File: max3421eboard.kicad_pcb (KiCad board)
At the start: 2 copper layers, 41 x 49 mm, 32 parts, among them J1 USB A, J2 USB MicroB, J3 1x10, J4 1x8, J5 1x8, J6 1x3, J7 Conn_01x04, U1 MAX3421E, U2 LP2985-3.3, U3 STMPS2141STR, Y1 12MHz

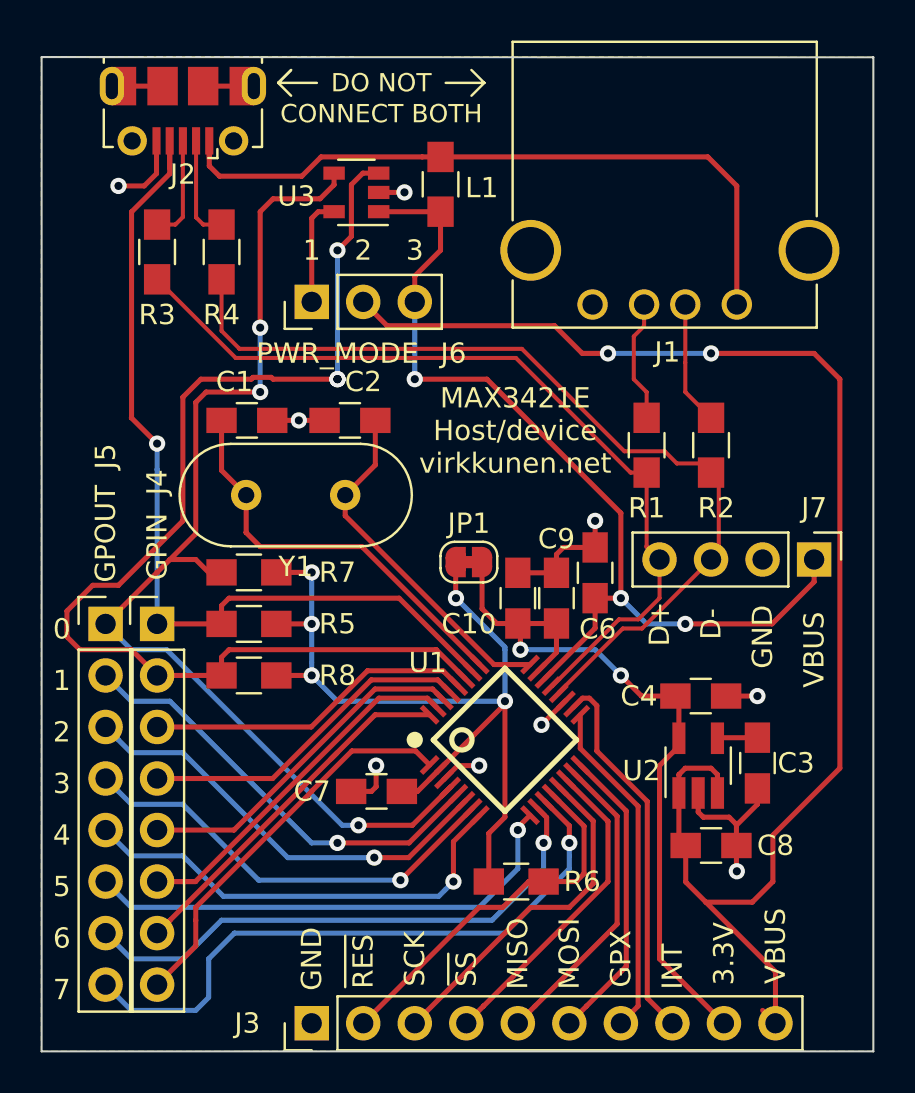
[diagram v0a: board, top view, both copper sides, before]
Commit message: Fix the board layout
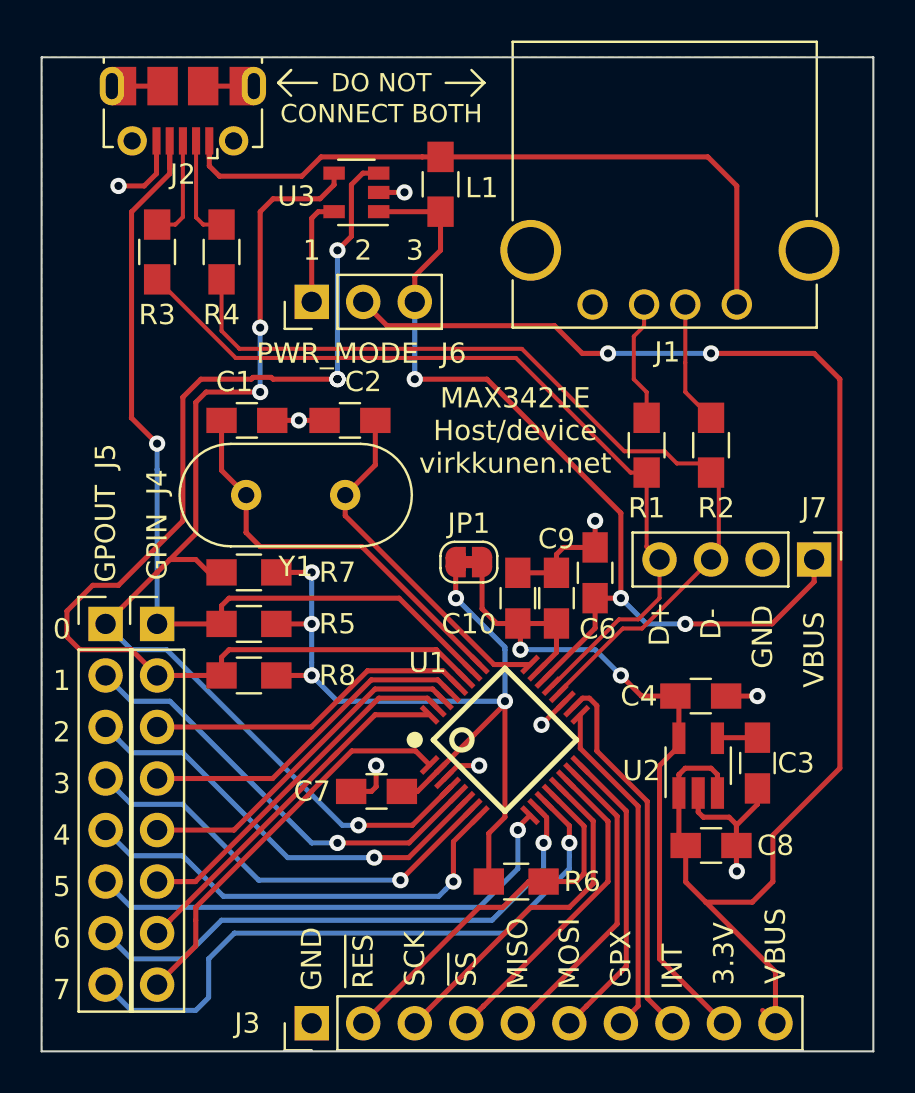
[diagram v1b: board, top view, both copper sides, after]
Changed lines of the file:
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@@
       (drillshape 0)
       (scaleselection 1)
-      (outputdirectory ""))
+      (outputdirectory "out-my/"))
   )
   (net 0 "")
@@
   )
   (gr_line (start 59 47) (end 59 96) (layer Edge.Cuts) (width 0.1))
-  (gr_line (start 18 46.99) (end 59 47) (layer Edge.Cuts) (width 0.1))
-  (gr_line (start 18 96) (end 18 46.99) (layer Edge.Cuts) (width 0.1))
+  (gr_line (start 18 47) (end 59 47) (layer Edge.Cuts) (width 0.1))
+  (gr_line (start 18 96) (end 18 47) (layer Edge.Cuts) (width 0.1))
   (segment (start 23.665 51.665) (end 23.695 51.435) (width 0.25) (layer F.Cu) (net 1))
   (segment (start 23.665 51.465) (end 23.695 51.435) (width 0.25) (layer F.Cu) (net 1))
@@
     (polygon
       (pts
-        (xy 59 96) (xy 18 96) (xy 18 46.99) (xy 59 47)
+        (xy 59 96) (xy 18 96) (xy 18 47) (xy 59 47)
       )
     )
